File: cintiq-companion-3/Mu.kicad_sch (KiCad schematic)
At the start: 12 parts, among them J1 Conn_01x03_Pin

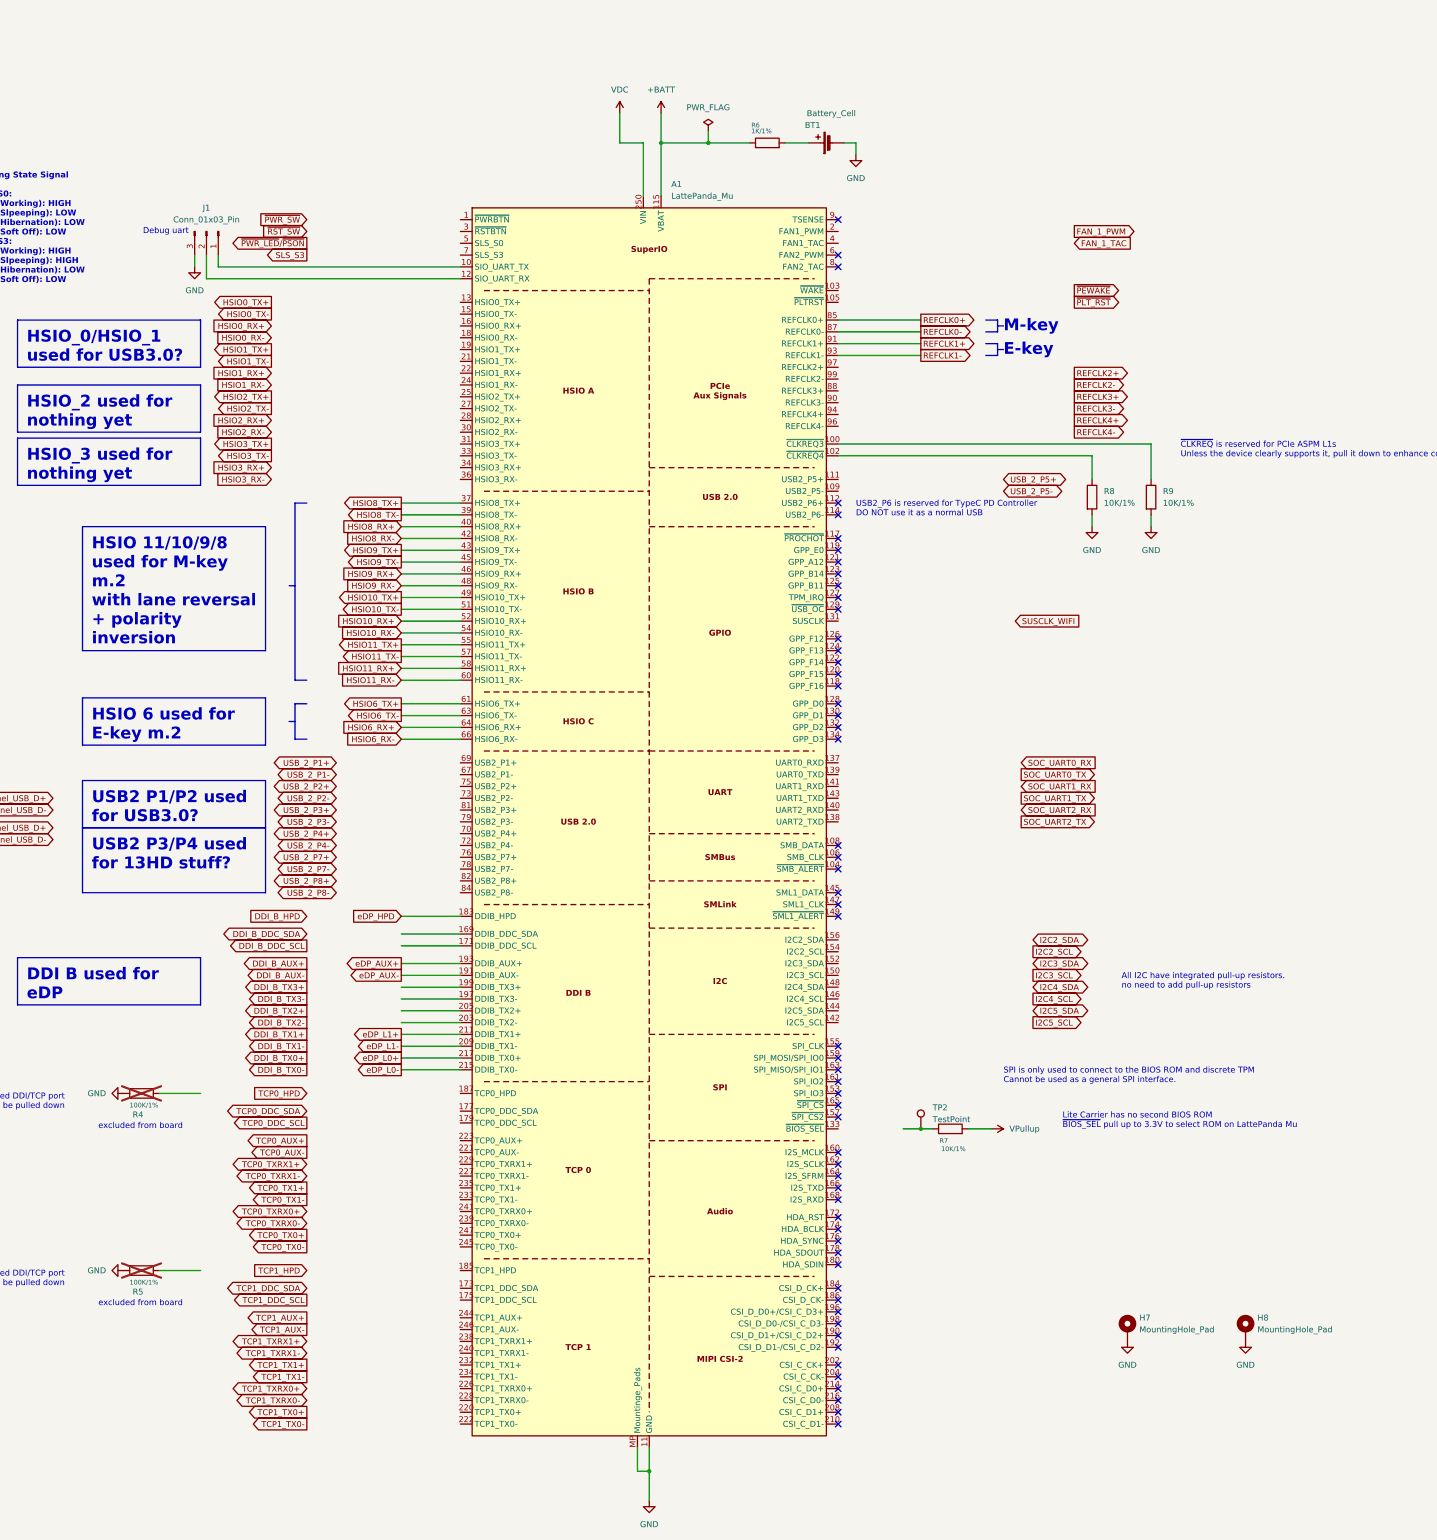
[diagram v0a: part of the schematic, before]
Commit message: susclk
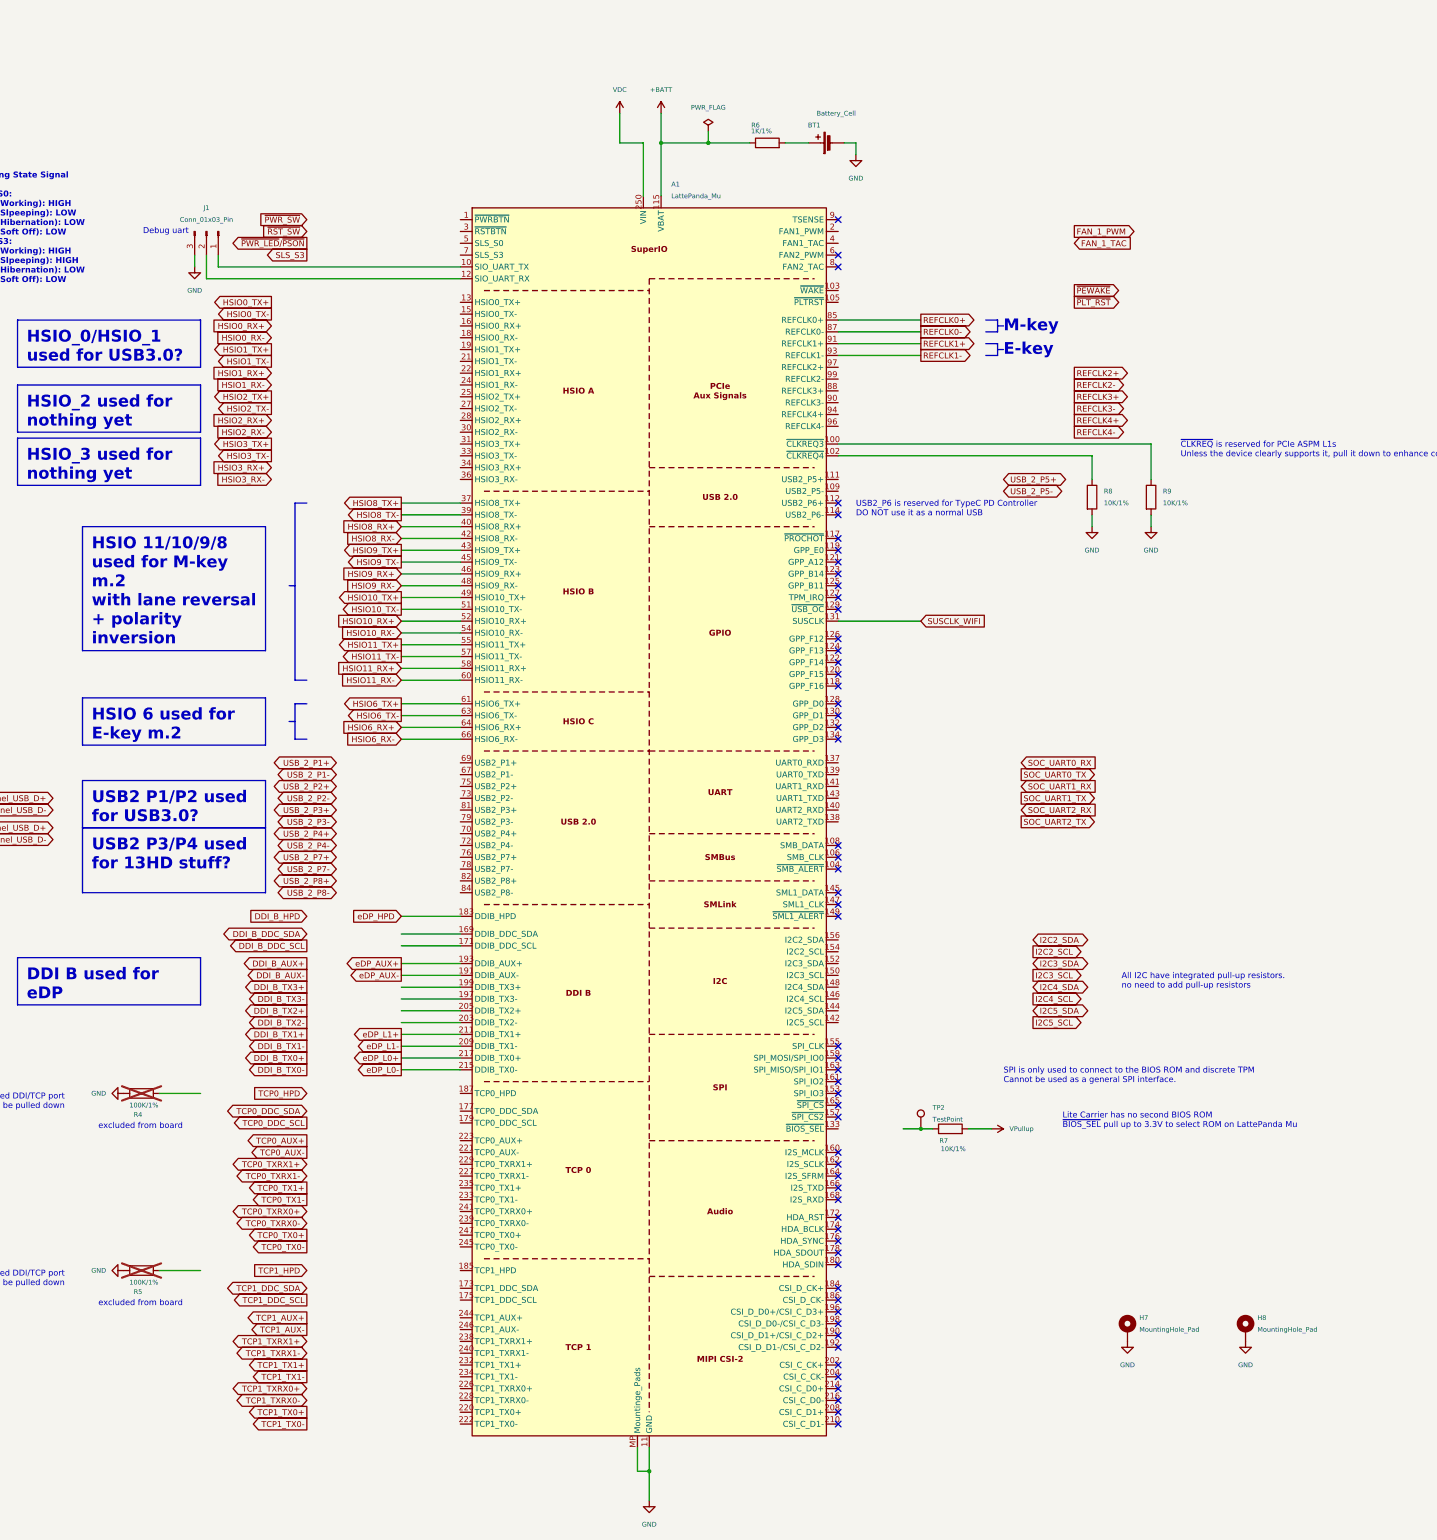
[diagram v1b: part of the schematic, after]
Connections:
- net SUSCLK_WIFI: now also A1.131 (SUSCLK)
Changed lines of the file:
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@@
 	(wire
 		(pts
+			(xy 427.99 158.75) (xy 445.77 158.75)
+		)
+		(stroke
+			(width 0)
+			(type default)
+		)
+	)
+	(wire
+		(pts
 			(xy 427.99 120.65) (xy 495.3 120.65)
 		)
@@
 	(global_label "SUSCLK_WIFI"
 		(shape input)
-		(at 466.09 158.75 0)
+		(at 445.77 158.75 0)
 		(fields_autoplaced yes)
 		(effects
@@
 		)
 		(property "Intersheetrefs" "${INTERSHEET_REFS}"
-			(at 466.09 158.75 0)
+			(at 445.77 158.75 0)
 			(effects
 				(font
@@
 			(effects
 				(font
-					(size 1.27 1.27)
+					(size 1.016 1.016)
 				)
 				(hide yes)
@@
 			(effects
 				(font
-					(size 1.27 1.27)
+					(size 1.016 1.016)
 				)
 			)
@@
 			(effects
 				(font
-					(size 1.27 1.27)
+					(size 1.016 1.016)
 				)
 			)
@@
 			(effects
 				(font
-					(size 1 1)
+					(size 1.016 1.016)
 				)
 			)
@@
 			(effects
 				(font
-					(size 1.27 1.27)
+					(size 1.016 1.016)
 				)
 				(hide yes)
@@
 			(effects
 				(font
-					(size 1.27 1.27)
+					(size 1.016 1.016)
 				)
 			)
@@
 			(effects
 				(font
-					(size 1.27 1.27)
+					(size 1.016 1.016)
 				)
 				(justify left)
@@
 			(effects
 				(font
-					(size 1.27 1.27)
+					(size 1.016 1.016)
 				)
 				(justify left)
@@
 			(effects
 				(font
-					(size 1.27 1.27)
+					(size 1.016 1.016)
 				)
 			)
@@
 			(effects
 				(font
-					(size 1 1)
+					(size 1.016 1.016)
 				)
 			)
@@
 			(effects
 				(font
-					(size 1.27 1.27)
+					(size 1.016 1.016)
 				)
 				(hide yes)
@@
 			(effects
 				(font
-					(size 1.27 1.27)
+					(size 1.016 1.016)
 				)
 			)
@@
 			(effects
 				(font
-					(size 1.27 1.27)
+					(size 1.016 1.016)
 				)
 				(justify left)
@@
 			(effects
 				(font
-					(size 1.27 1.27)
+					(size 1.016 1.016)
 				)
 				(justify left)
@@
 			(effects
 				(font
-					(size 1.27 1.27)
+					(size 1.016 1.016)
 				)
 				(hide yes)
@@
 			(effects
 				(font
-					(size 1.27 1.27)
+					(size 1.016 1.016)
 				)
 				(justify left)
@@
 			(effects
 				(font
-					(size 1.27 1.27)
+					(size 1.016 1.016)
 				)
 				(justify left)
@@
 			(effects
 				(font
-					(size 1.27 1.27)
+					(size 1.016 1.016)
 				)
 				(justify left)
@@
 			(effects
 				(font
-					(size 1.27 1.27)
+					(size 1.016 1.016)
 				)
 				(hide yes)
@@
 			(effects
 				(font
-					(size 1.27 1.27)
+					(size 1.016 1.016)
 				)
 			)
@@
 			(effects
 				(font
-					(size 1.27 1.27)
+					(size 1.016 1.016)
 				)
 				(justify left)
@@
 			(effects
 				(font
-					(size 1.27 1.27)
+					(size 1.016 1.016)
 				)
 				(justify left)
@@
 			(effects
 				(font
-					(size 1.27 1.27)
+					(size 1.016 1.016)
 				)
 				(justify left)
@@
 			(effects
 				(font
-					(size 1.27 1.27)
+					(size 1.016 1.016)
 				)
 				(justify left)
@@
 			(effects
 				(font
-					(size 1 1)
+					(size 1.016 1.016)
 				)
 			)
@@
 			(effects
 				(font
-					(size 1 1)
+					(size 1.016 1.016)
 				)
 			)
@@
 			(effects
 				(font
-					(size 1.27 1.27)
+					(size 1.016 1.016)
 				)
 				(hide yes)
@@
 			(effects
 				(font
-					(size 1.27 1.27)
+					(size 1.016 1.016)
 				)
 				(justify right)
@@
 			(effects
 				(font
-					(size 1.27 1.27)
+					(size 1.016 1.016)
 				)
 				(hide yes)
@@
 			(effects
 				(font
-					(size 1.27 1.27)
+					(size 1.016 1.016)
 				)
 				(justify right)
@@
 			(effects
 				(font
-					(size 1.27 1.27)
+					(size 1.016 1.016)
 				)
 				(hide yes)
@@
 			(effects
 				(font
-					(size 1.27 1.27)
+					(size 1.016 1.016)
 				)
 			)
@@
 			(effects
 				(font
-					(size 1.27 1.27)
+					(size 1.016 1.016)
 				)
 				(hide yes)
@@
 			(effects
 				(font
-					(size 1.27 1.27)
+					(size 1.016 1.016)
 				)
 			)
@@
 			(effects
 				(font
-					(size 1 1)
+					(size 1.016 1.016)
 				)
 				(justify left)
@@
 			(effects
 				(font
-					(size 1 1)
+					(size 1.016 1.016)
 				)
 				(justify left)
@@
 			(effects
 				(font
-					(size 1.27 1.27)
+					(size 1.016 1.016)
 				)
 				(hide yes)
@@
 			(effects
 				(font
-					(size 1.27 1.27)
+					(size 1.016 1.016)
 				)
 			)
@@
 			(effects
 				(font
-					(size 1.27 1.27)
+					(size 1.016 1.016)
 				)
 				(hide yes)
@@
 			(effects
 				(font
-					(size 1.27 1.27)
+					(size 1.016 1.016)
 				)
 			)
@@
 			(effects
 				(font
-					(size 1.27 1.27)
+					(size 1.016 1.016)
 				)
 				(hide yes)
@@
 			(effects
 				(font
-					(size 1.27 1.27)
+					(size 1.016 1.016)
 				)
 			)
@@
 			(effects
 				(font
-					(size 1.27 1.27)
+					(size 1.016 1.016)
 				)
 				(justify left)
@@
 			(effects
 				(font
-					(size 1.27 1.27)
+					(size 1.016 1.016)
 				)
 				(justify left)
@@
 			(effects
 				(font
-					(size 1.27 1.27)
+					(size 1.016 1.016)
 				)
 				(hide yes)
@@
 			(effects
 				(font
-					(size 1.27 1.27)
+					(size 1.016 1.016)
 				)
 			)
@@
 			(effects
 				(font
-					(size 1.27 1.27)
+					(size 1.016 1.016)
 				)
 				(justify left)
@@
 			(effects
 				(font
-					(size 1.27 1.27)
+					(size 1.016 1.016)
 				)
 				(justify left)
@@
 			(effects
 				(font
-					(size 1.27 1.27)
+					(size 1.016 1.016)
 				)
 			)
@@
 			(effects
 				(font
-					(size 1.27 1.27)
+					(size 1.016 1.016)
 				)
 			)
